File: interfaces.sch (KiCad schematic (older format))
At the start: 25 parts

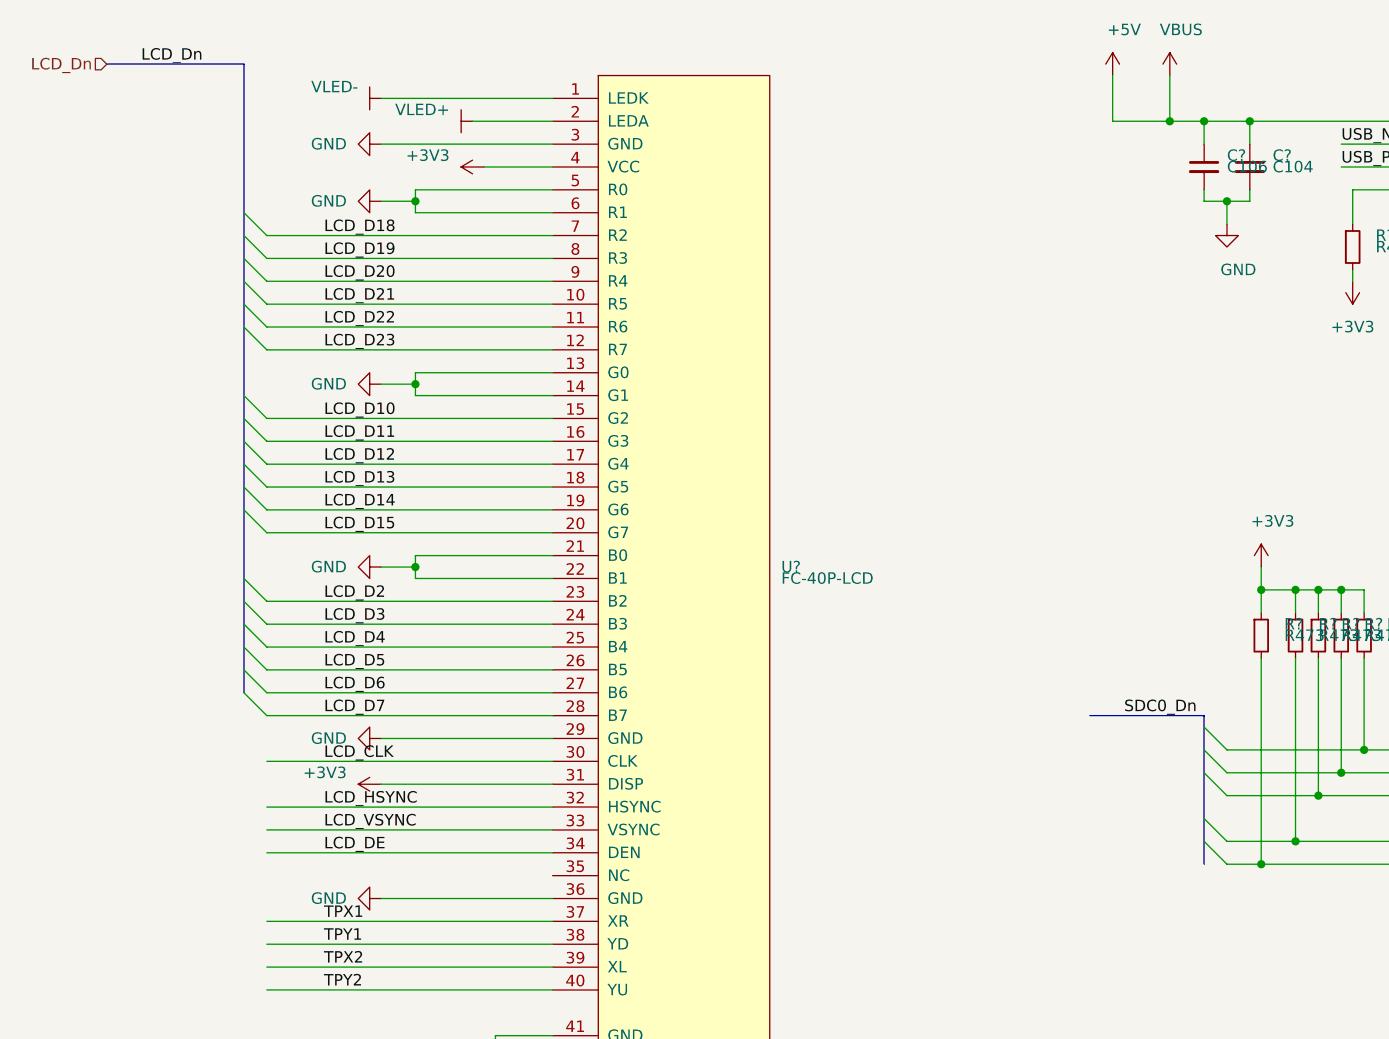
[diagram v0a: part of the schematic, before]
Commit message: update,
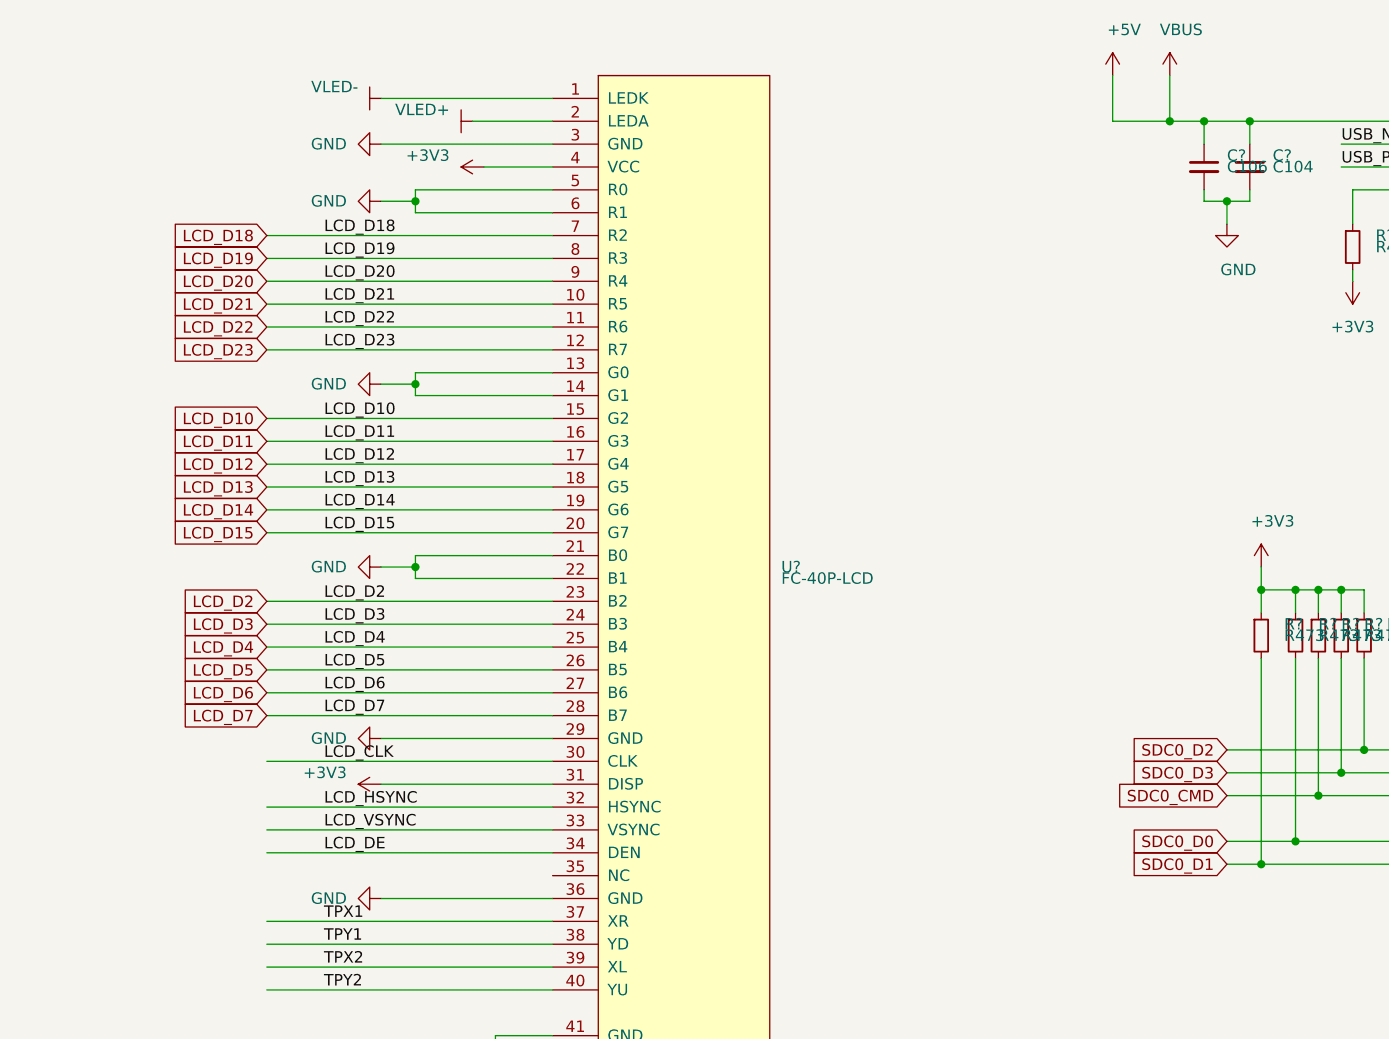
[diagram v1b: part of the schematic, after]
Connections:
- net labels removed: LCD_Dn, SDC0_Dn
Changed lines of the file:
@@
 EESchema Schematic File Version 4
-LIBS:I2C-adc-cache
+LIBS:allwinner-v3s-tryout-cache
 EELAYER 26 0
 EELAYER END
@@
 Wire Wire Line
 	8350 6400 8200 6400
-Wire Bus Line
-	5250 5600 5750 5600
-Text Label 5400 5600 0    50   ~ 0
-SDC0_Dn
 Text Label 6650 5750 0    50   ~ 0
 SDC0_D2
@@
 Text Label 6650 6250 0    50   ~ 0
 SDC0_D1
-Entry Wire Line
-	5850 6250 5750 6150
-Entry Wire Line
-	5750 6050 5850 6150
-Entry Wire Line
-	5750 5850 5850 5950
-Entry Wire Line
-	5750 5750 5850 5850
-Entry Wire Line
-	5750 5650 5850 5750
 Wire Wire Line
 	7100 5750 6450 5750
@@
 Wire Wire Line
 	10500 3450 10850 3450
-Entry Wire Line
-	1550 5500 1650 5600
-Entry Wire Line
-	1550 5400 1650 5500
-Entry Wire Line
-	1550 5300 1650 5400
-Entry Wire Line
-	1550 5200 1650 5300
-Entry Wire Line
-	1550 5100 1650 5200
-Entry Wire Line
-	1550 5000 1650 5100
-Entry Wire Line
-	1550 4700 1650 4800
-Entry Wire Line
-	1550 4600 1650 4700
-Entry Wire Line
-	1550 4500 1650 4600
-Entry Wire Line
-	1550 4400 1650 4500
-Entry Wire Line
-	1550 4300 1650 4400
-Entry Wire Line
-	1550 4200 1650 4300
-Entry Wire Line
-	1550 3900 1650 4000
-Entry Wire Line
-	1550 3800 1650 3900
-Entry Wire Line
-	1550 3700 1650 3800
-Entry Wire Line
-	1550 3600 1650 3700
-Entry Wire Line
-	1550 3500 1650 3600
-Entry Wire Line
-	1550 3400 1650 3500
-Wire Bus Line
-	1550 2750 950  2750
-Text Label 1100 2750 0    50   ~ 0
-LCD_Dn
 $Comp
 L customized_power:+3V3 #PWR?
@@
 Wire Wire Line
 	8350 9000 8350 9350
-Wire Bus Line
-	1550 2750 1550 5500
-Wire Bus Line
-	5750 5600 5750 6250
-Text HLabel 950  2750 0    50   Input ~ 0
-LCD_Dn
+Text GLabel 1650 3500 0    50   Input ~ 0
+LCD_D18
+Text GLabel 1650 3600 0    50   Input ~ 0
+LCD_D19
+Text GLabel 1650 3700 0    50   Input ~ 0
+LCD_D20
+Text GLabel 1650 3800 0    50   Input ~ 0
+LCD_D21
+Text GLabel 1650 3900 0    50   Input ~ 0
+LCD_D22
+Text GLabel 1650 4000 0    50   Input ~ 0
+LCD_D23
+Text GLabel 1650 4300 0    50   Input ~ 0
+LCD_D10
+Text GLabel 1650 4400 0    50   Input ~ 0
+LCD_D11
+Text GLabel 1650 4500 0    50   Input ~ 0
+LCD_D12
+Text GLabel 1650 4600 0    50   Input ~ 0
+LCD_D13
+Text GLabel 1650 4700 0    50   Input ~ 0
+LCD_D14
+Text GLabel 1650 4800 0    50   Input ~ 0
+LCD_D15
+Text GLabel 1650 5100 0    50   Input ~ 0
+LCD_D2
+Text GLabel 1650 5200 0    50   Input ~ 0
+LCD_D3
+Text GLabel 1650 5300 0    50   Input ~ 0
+LCD_D4
+Text GLabel 1650 5400 0    50   Input ~ 0
+LCD_D5
+Text GLabel 1650 5500 0    50   Input ~ 0
+LCD_D6
+Text GLabel 1650 5600 0    50   Input ~ 0
+LCD_D7
+Text GLabel 5850 5750 0    50   Input ~ 0
+SDC0_D2
+Text GLabel 5850 5850 0    50   Input ~ 0
+SDC0_D3
+Text GLabel 5850 5950 0    50   Input ~ 0
+SDC0_CMD
+Text GLabel 5850 6150 0    50   Input ~ 0
+SDC0_D0
+Text GLabel 5850 6250 0    50   Input ~ 0
+SDC0_D1
 $EndSCHEMATC

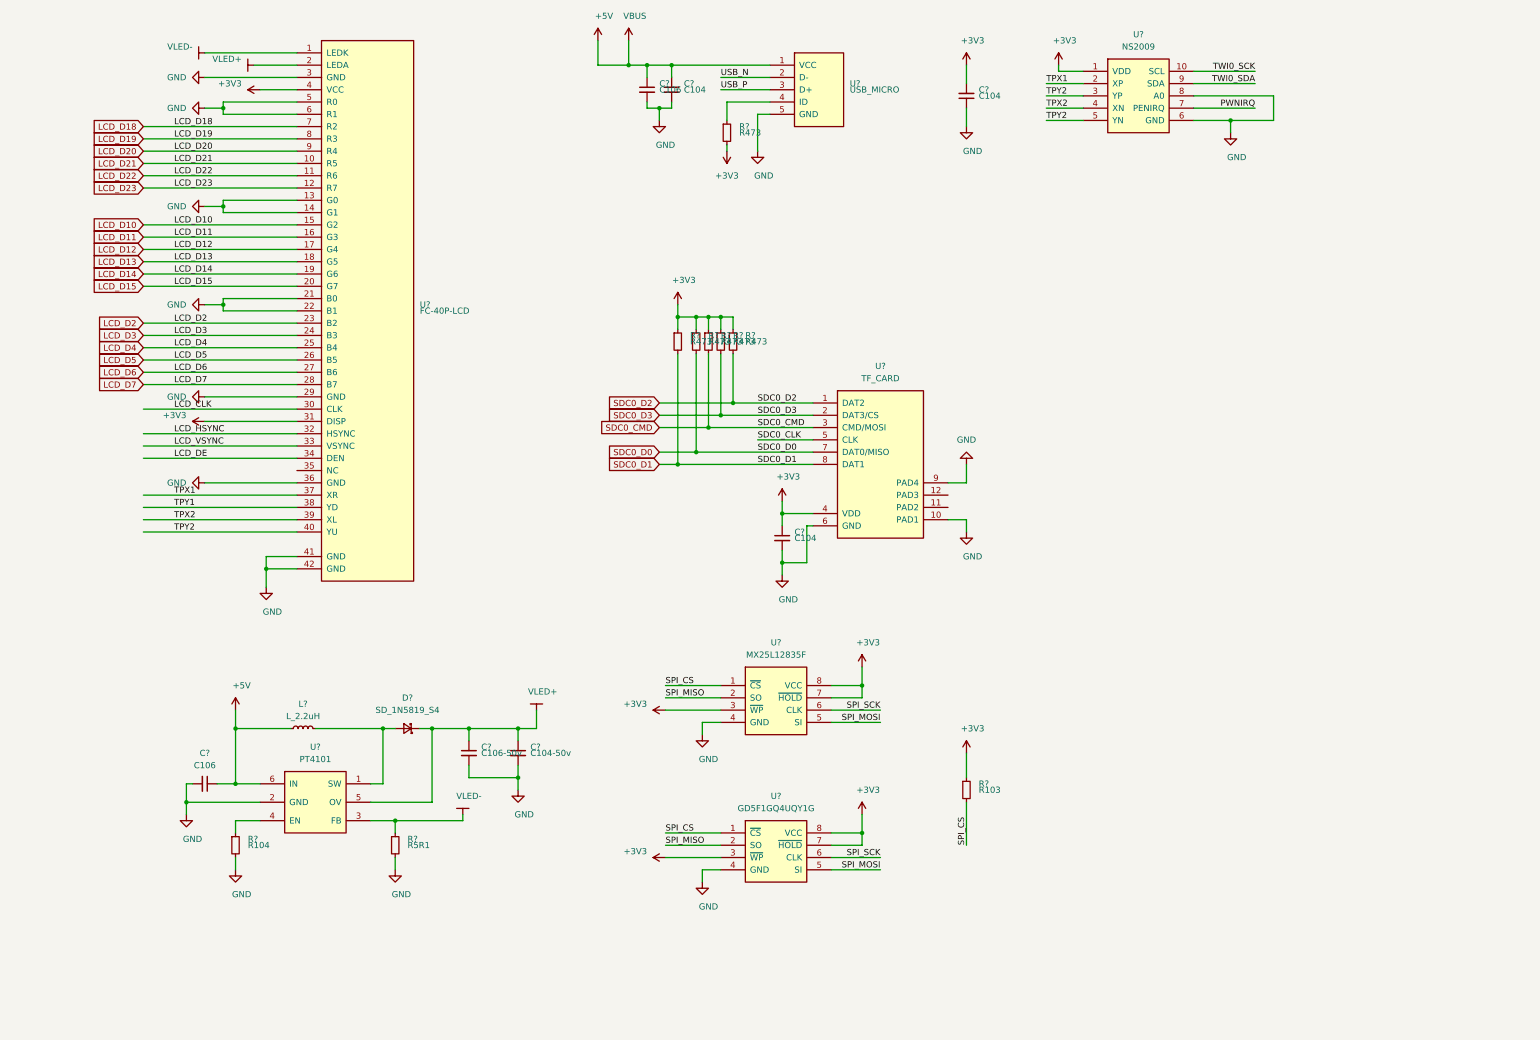
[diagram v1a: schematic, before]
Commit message: update,
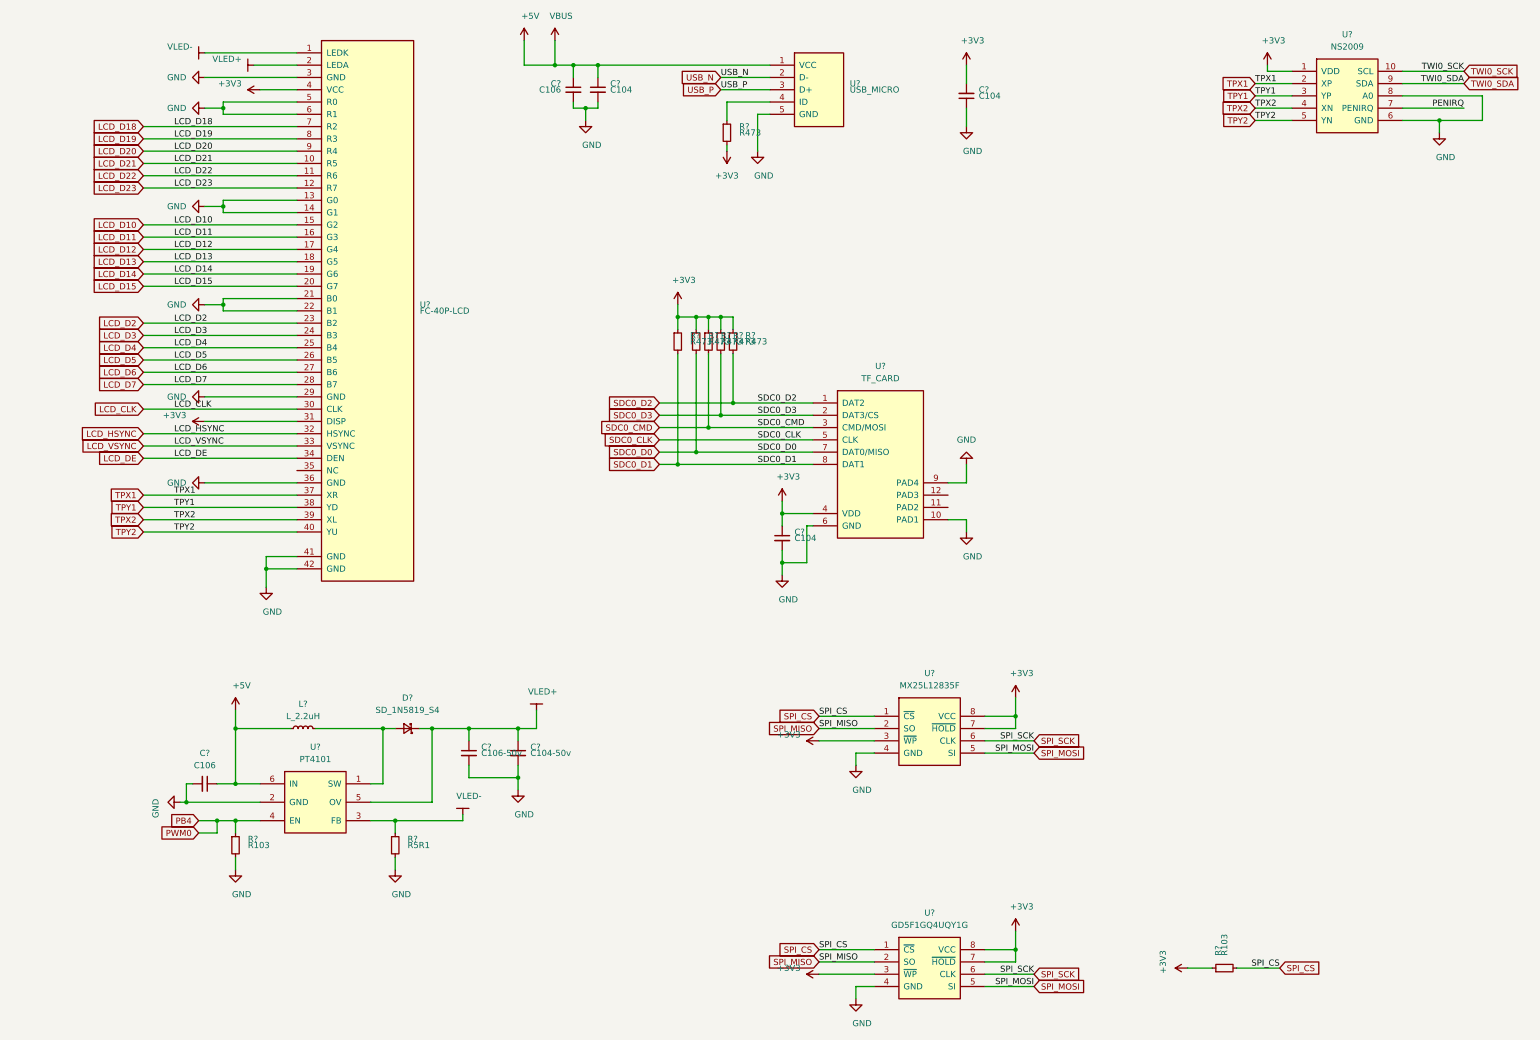
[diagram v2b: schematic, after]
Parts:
- R?: value R104 -> R103
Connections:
- net labels added: PB4, PENIRQ, PWM0
- net labels removed: PWNIRQ
- wire segments 184 -> 188
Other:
- moved on the sheet: C?, R?, U?
